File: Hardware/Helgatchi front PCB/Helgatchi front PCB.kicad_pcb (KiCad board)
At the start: 2 copper layers, 100.2 x 80 mm, 43 parts, among them J1 BATTERY, J2 SCREEN, J3 SMA, J4 u.FL, M1 MOTOR, Q1 NMOS, SW1 LEFT BUTTON, SW2 CENTER BUTTON, SW3 RIGHT BUTTON, U1 XIAO ESP32-S3

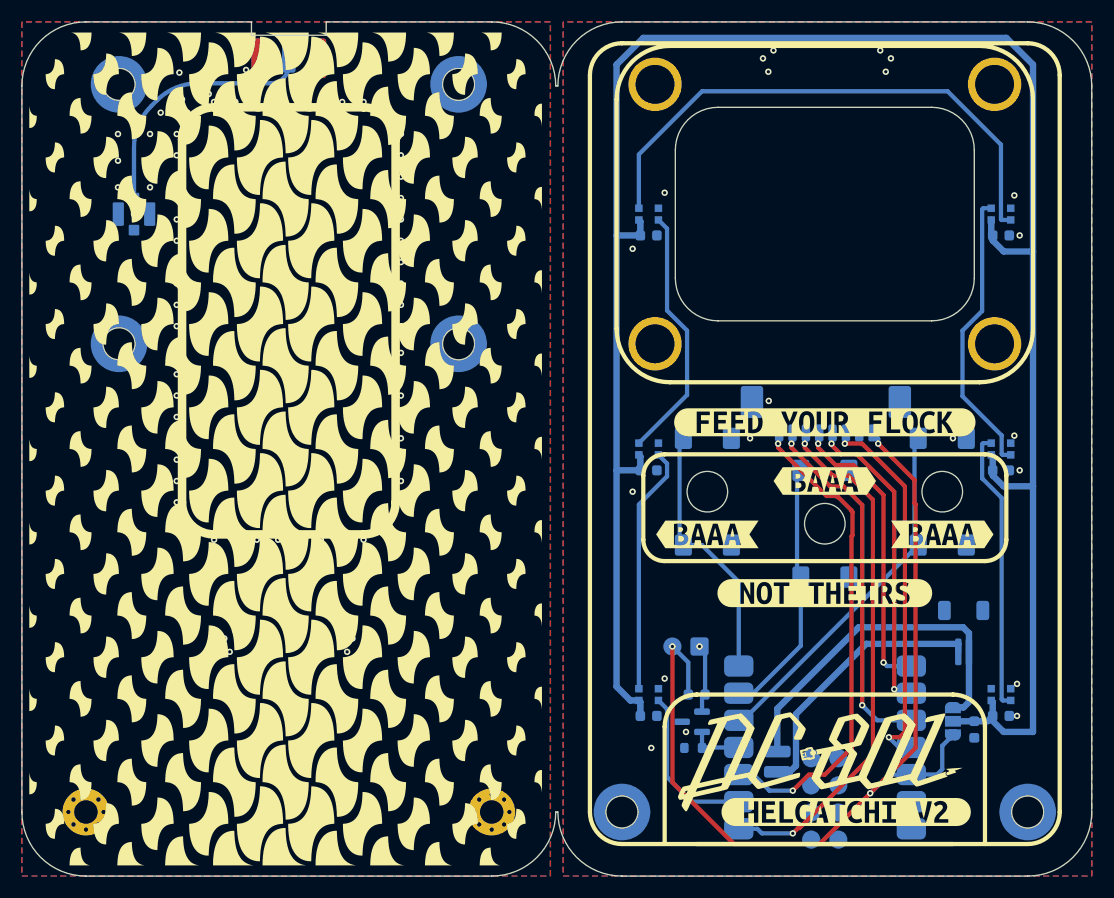
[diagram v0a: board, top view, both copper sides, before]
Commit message: slopsoftware
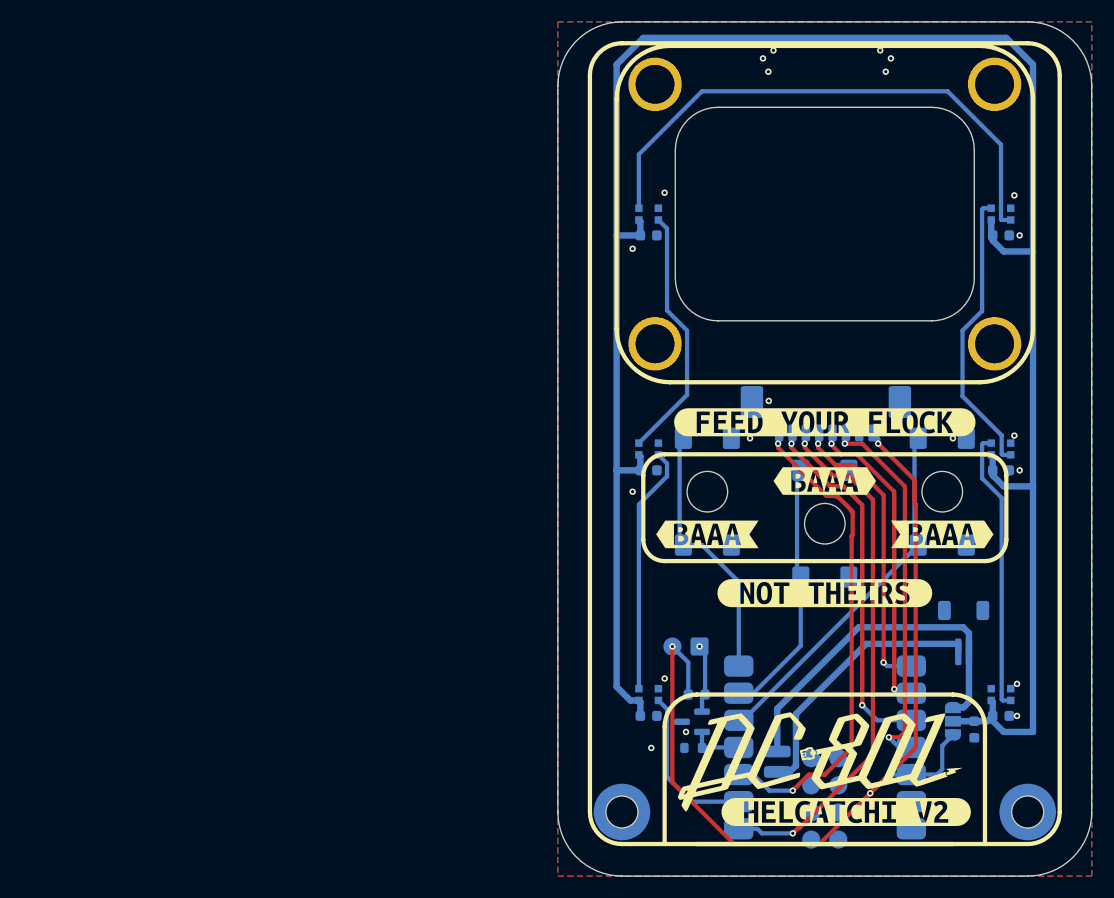
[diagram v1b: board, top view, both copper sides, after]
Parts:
- removed the G*** at (113.5, 98.5)
- removed the H2 at (129.7, 64.3)
- removed the H2 at (129.7, 88.7)
- removed the H2 at (97.9, 88.7)
- removed the H2 at (97.9, 64.3)
- removed J3: SMA, Connector_Coaxial:SMA_Samtec_SMA-J-P-H-ST-EM1_EdgeMount
- removed J4: u.FL, Connector_Coaxial:U.FL_Molex_MCRF_73412-0110_Vertical
- removed REF** (x2): MountingHole_2.2mm_M2_Pad_Via, MountingHole:MountingHole_2.2mm_M2_Pad_Via
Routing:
- net Net-(J3-In): track 24.4 -> 0.00 mm
- net (no net): track 29.1 -> 14.5 mm, vias 12 -> 6
- net GND: vias 90 -> 15
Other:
- board size 100.2 x 80 mm -> 50 x 80 mm
- board text removed: "2.4GHZ ANTENNA"
- board text removed: "CREDITS"
- board text removed: "Netkisune Poly801 kimb3r n1ghtbl00d Wade"
